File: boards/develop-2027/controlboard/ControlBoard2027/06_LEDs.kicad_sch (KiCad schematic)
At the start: 17 parts, among them U7 74AHCT125

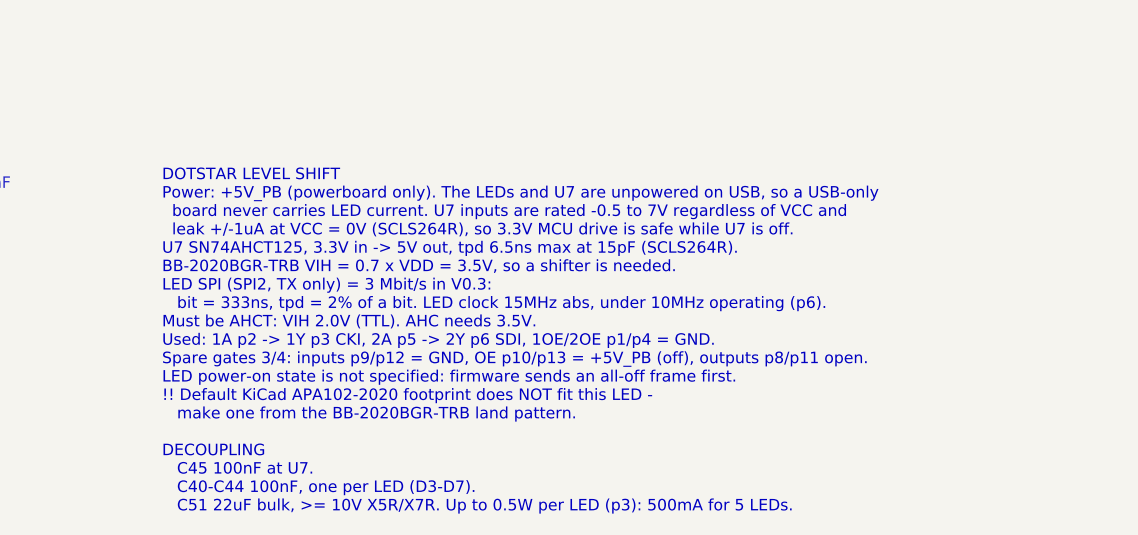
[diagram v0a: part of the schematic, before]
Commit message: Updated comments. Claude did an audit. Take it with huge grains of salt
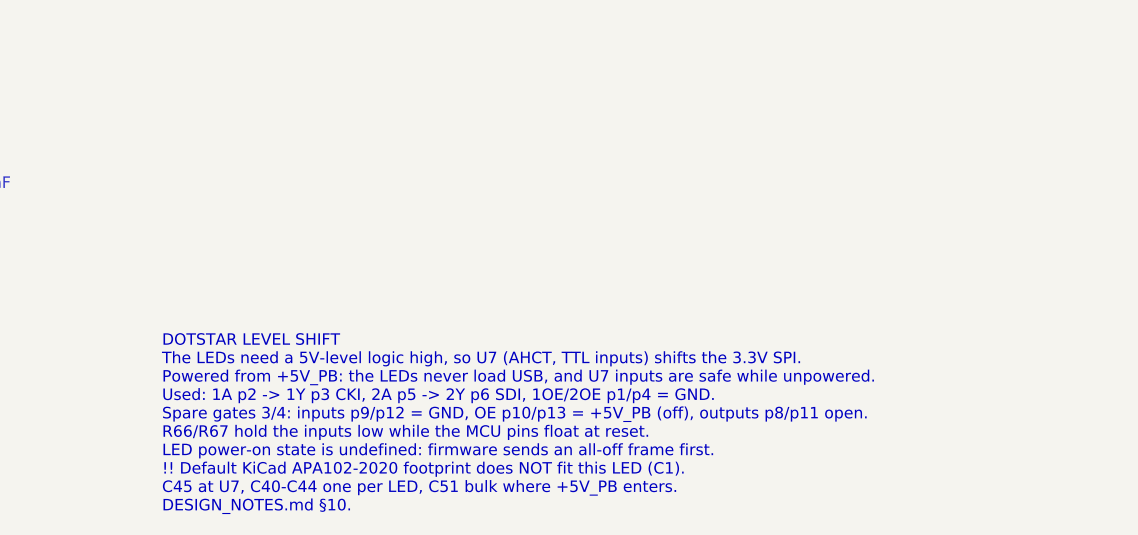
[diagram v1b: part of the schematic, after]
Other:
- note added: "DOTSTAR LEVEL SHIFT The LEDs need a 5V-level logic high, so U7 (AHCT, TTL inputs) shifts the 3.3V SPI. Powered from +5V_PB: the LEDs never load USB, and U7 inputs are safe while unpowered. Used: 1A p2 -> 1Y p3 CKI, 2A p5 -> 2Y p6 SDI, 1OE/2OE p1/p4 = GND. Spare gates 3/4: inputs p9/p12 = GND, OE p10/p13 = +5V_PB (off), outputs p8/p11 open. R66/R67 hold the inputs low while the MCU pins float at r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"
- note removed: "DOTSTAR LEVEL SHIFT Power: +5V_PB (powerboard only). The LEDs and U7 are unpowered on USB, so a USB-only board never carries LED current. U7 inputs are rated -0.5 to 7V regardless of VCC and leak +/-1uA at VCC = 0V (SCLS264R), so 3.3V MCU drive is safe while U7 is off. U7 SN74AHCT125, 3.3V in -> 5V out, tpd 6.5ns max at 15pF (SCLS264R). BB-2020BGR-TRB VIH = 0.7 x VDD = 3.5V, so a shifter is neede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"
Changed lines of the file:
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@@
     (effects (font (size 1.27 1.27) (bold yes) (color 255 0 0 1)) (justify left bottom))
   )
-  (text "DOTSTAR LEVEL SHIFT\nPower: +5V_PB (powerboard only). The LEDs and U7 are unpowered on USB, so a USB-only\n  board never carries LED current. U7 inputs are rated -0.5 to 7V regardless of VCC and\n  leak +/-1uA at VCC = 0V (SCLS264R), so 3.3V MCU drive is safe while U7 is off.\nU7 SN74AHCT125, 3.3V in -> 5V out, tpd 6.5ns max at 15pF (SCLS264R).\nBB-2020BGR-TRB VIH = 0.7 x VDD = 3.5V, so a shifter is needed.\nLED SPI (SPI2, TX only) = 3 Mbit/s in V0.3:\n   bit = 333ns, tpd = 2% of a bit. LED clock 15MHz abs, under 10MHz operating (p6).\nMust be AHCT: VIH 2.0V (TTL). AHC needs 3.5V.\nUsed: 1A p2 -> 1Y p3 CKI, 2A p5 -> 2Y p6 SDI, 1OE/2OE p1/p4 = GND.\nSpare gates 3/4: inputs p9/p12 = GND, OE p10/p13 = +5V_PB (off), outputs p8/p11 open.\nLED power-on state is not specified: firmware sends an all-off frame first.\n!! Default KiCad APA102-2020 footprint does NOT fit this LED -\n   make one from the BB-2020BGR-TRB land pattern.\n\nDECOUPLING\n   C45 100nF at U7.\n   C40-C44 100nF, one per LED (D3-D7).\n   C51 22uF bulk, >= 10V X5R/X7R. Up to 0.5W per LED (p3): 500mA for 5 LEDs."
+  (text "DOTSTAR LEVEL SHIFT\nThe LEDs need a 5V-level logic high, so U7 (AHCT, TTL inputs) shifts the 3.3V SPI.\nPowered from +5V_PB: the LEDs never load USB, and U7 inputs are safe while unpowered.\nUsed: 1A p2 -> 1Y p3 CKI, 2A p5 -> 2Y p6 SDI, 1OE/2OE p1/p4 = GND.\nSpare gates 3/4: inputs p9/p12 = GND, OE p10/p13 = +5V_PB (off), outputs p8/p11 open.\nR66/R67 hold the inputs low while the MCU pins float at reset.\nLED power-on state is undefined: firmware sends an all-off frame first.\n!! Default KiCad APA102-2020 footprint does NOT fit this LED (C1).\nC45 at U7, C40-C44 one per LED, C51 bulk where +5V_PB enters.\nDESIGN_NOTES.md §10."
     (at 297.18 252.73 0)
     (effects (font (size 1.27 1.27)) (justify left bottom))

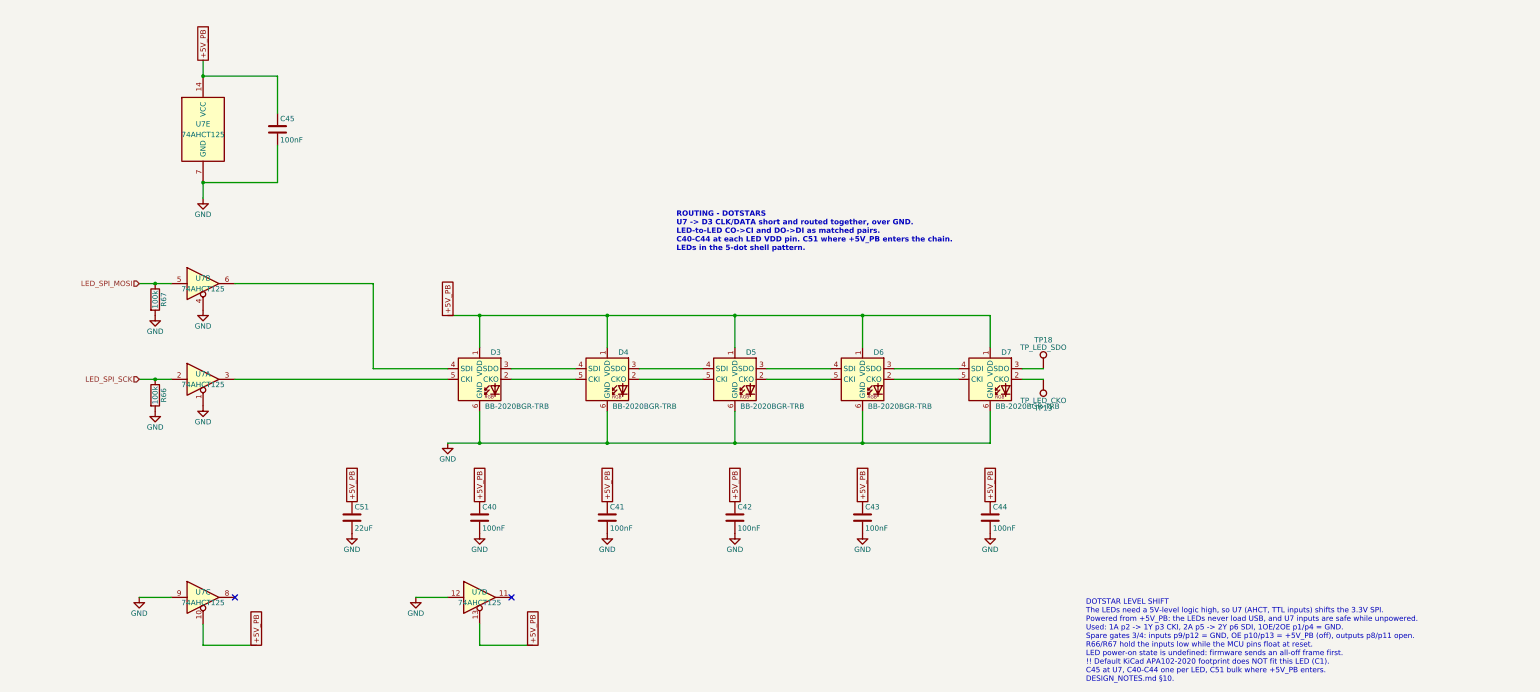
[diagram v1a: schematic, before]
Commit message: boxing goes brrr
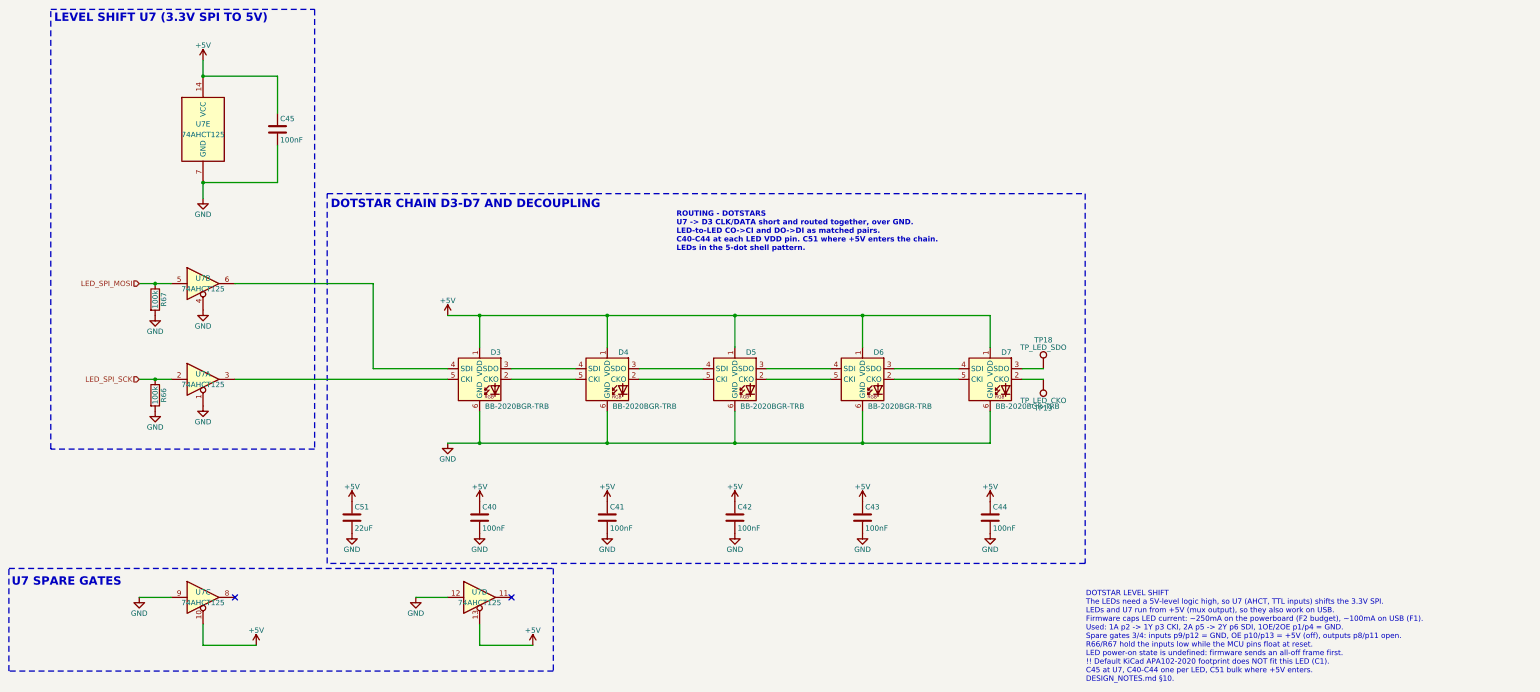
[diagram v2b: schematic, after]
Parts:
- U7: MPN (none) -> TI SN74AHCT125PWR
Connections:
- net +5V_PB renamed +5V
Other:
- note added: "DOTSTAR CHAIN D3-D7 AND DECOUPLING"
- note added: "DOTSTAR LEVEL SHIFT The LEDs need a 5V-level logic high, so U7 (AHCT, TTL inputs) shifts the 3.3V SPI. LEDs and U7 run from +5V (mux output), so they also work on USB. Firmware caps LED current: ~250mA on the powerboard (F2 budget), ~100mA on USB (F1). Used: 1A p2 -> 1Y p3 CKI, 2A p5 -> 2Y p6 SDI, 1OE/2OE p1/p4 = GND. Spare gates 3/4: inputs p9/p12 = GND, OE p10/p13 = +5V (off), outputs p8/p11 op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"
- note added: "LEVEL SHIFT U7 (3.3V SPI TO 5V)"
- note added: "ROUTING - DOTSTARS U7 -> D3 CLK/DATA short and routed together, over GND. LED-to-LED CO->CI and DO->DI as matched pairs. C40-C44 at each LED VDD pin. C51 where +5V enters the chain. LEDs in the 5-dot shell pattern."
- note added: "U7 SPARE GATES"
- note removed: "DOTSTAR LEVEL SHIFT The LEDs need a 5V-level logic high, so U7 (AHCT, TTL inputs) shifts the 3.3V SPI. Powered from +5V_PB: the LEDs never load USB, and U7 inputs are safe while unpowered. Used: 1A p2 -> 1Y p3 CKI, 2A p5 -> 2Y p6 SDI, 1OE/2OE p1/p4 = GND. Spare gates 3/4: inputs p9/p12 = GND, OE p10/p13 = +5V_PB (off), outputs p8/p11 open. R66/R67 hold the inputs low while the MCU pins float at r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"
- note removed: "ROUTING - DOTSTARS U7 -> D3 CLK/DATA short and routed together, over GND. LED-to-LED CO->CI and DO->DI as matched pairs. C40-C44 at each LED VDD pin. C51 where +5V_PB enters the chain. LEDs in the 5-dot shell pattern."
